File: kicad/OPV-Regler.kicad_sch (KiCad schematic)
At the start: 17 parts, among them U1 TL081, U2 TL081, U3 TL081, U4 TL081, U5 TL081

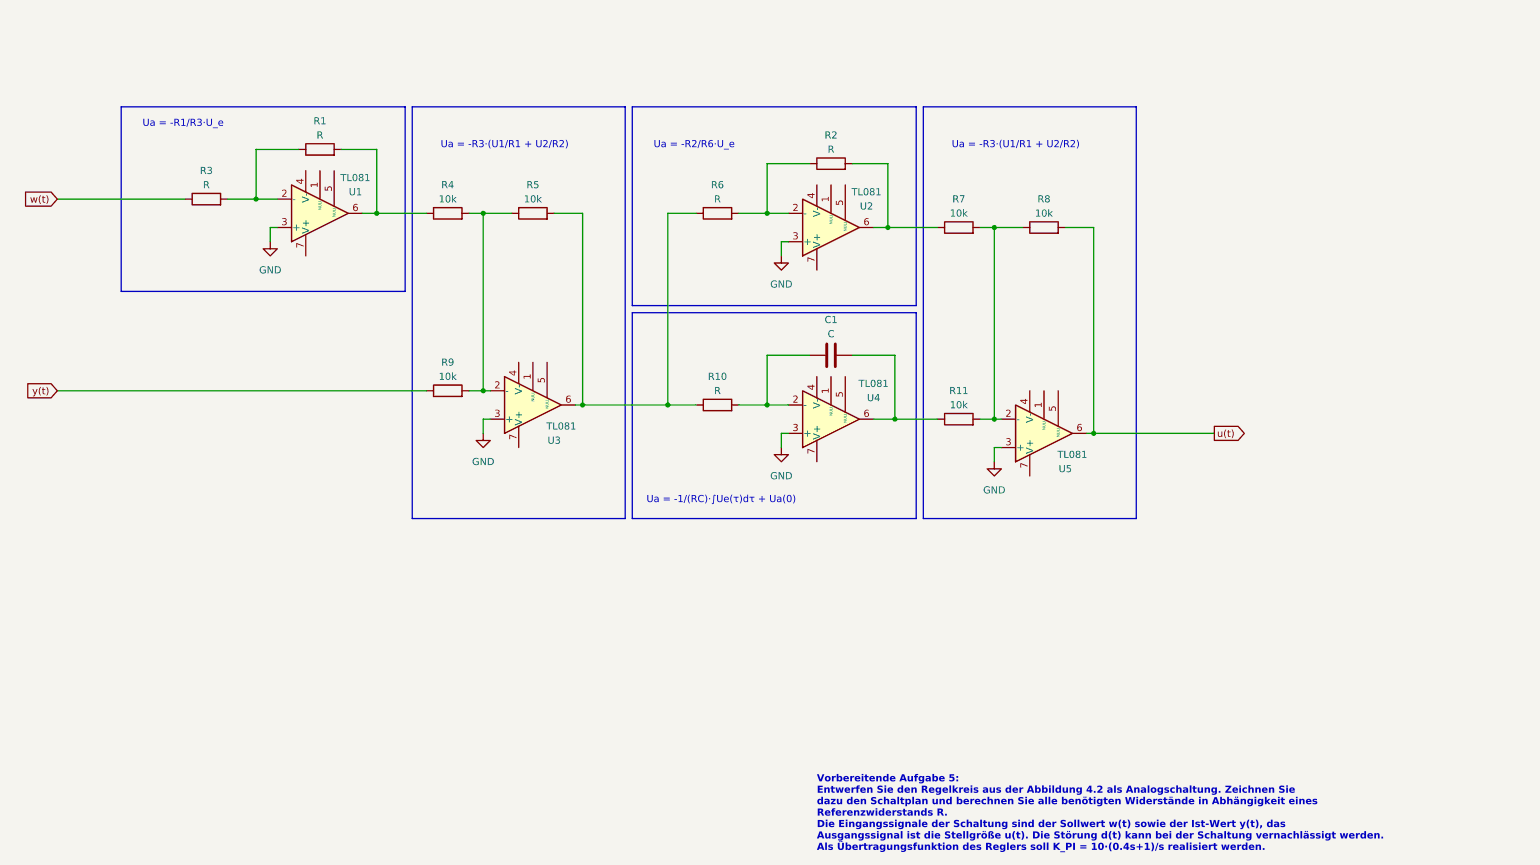
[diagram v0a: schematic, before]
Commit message: Add schaltplan pdf
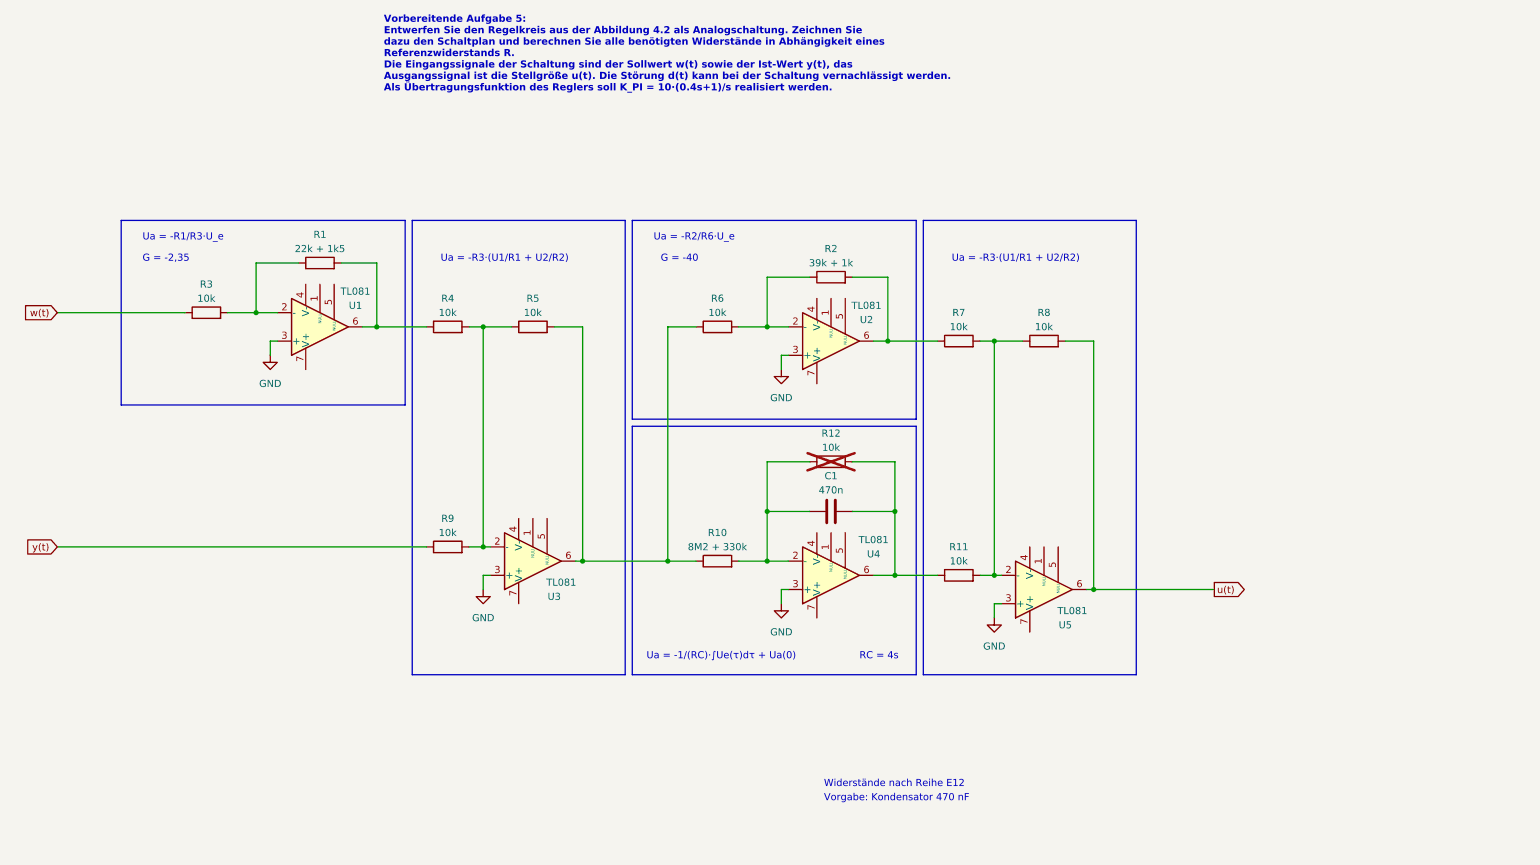
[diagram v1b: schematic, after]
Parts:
- added R12: 10k, symbol Device:R
- C1: value C -> 470n
- R1: value R -> 22k + 1k5
- R10: value R -> 8M2 + 330k
- R2: value R -> 39k + 1k
- R3, R6: value R -> 10k
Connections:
- net at C1.1, R10.2, U4.2 (-): now also R12.1
- net at C1.2, R11.1, U4.6: now also R12.2
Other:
- note added: "G = -2,35"
- note added: "G = -40"
- note added: "RC = 4s"
- note added: "Vorgabe: Kondensator 470 nF"
- note added: "Widerstände nach Reihe E12"
- company: (none) -> Universität Ulm
- title: (none) -> ERT-Praktikum - Aufgabe 5: PI-Regler
- moved on the sheet: C1, R1, R10, R11, R2, R3, R4, R5, R6, R7, R8, R9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
